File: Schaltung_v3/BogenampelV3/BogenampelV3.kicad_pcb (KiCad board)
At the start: 2 copper layers, 89 x 36 mm, 50 parts, among them IC1 TPS62742DSSR, J1 Conn_01x24_Pin, Q1 IRLML9301, Q2 IRLML6346, Q3 Si1308EDL, SW1 SW_Push, SW2 SW_Push, U1 XIAO ESP32C3

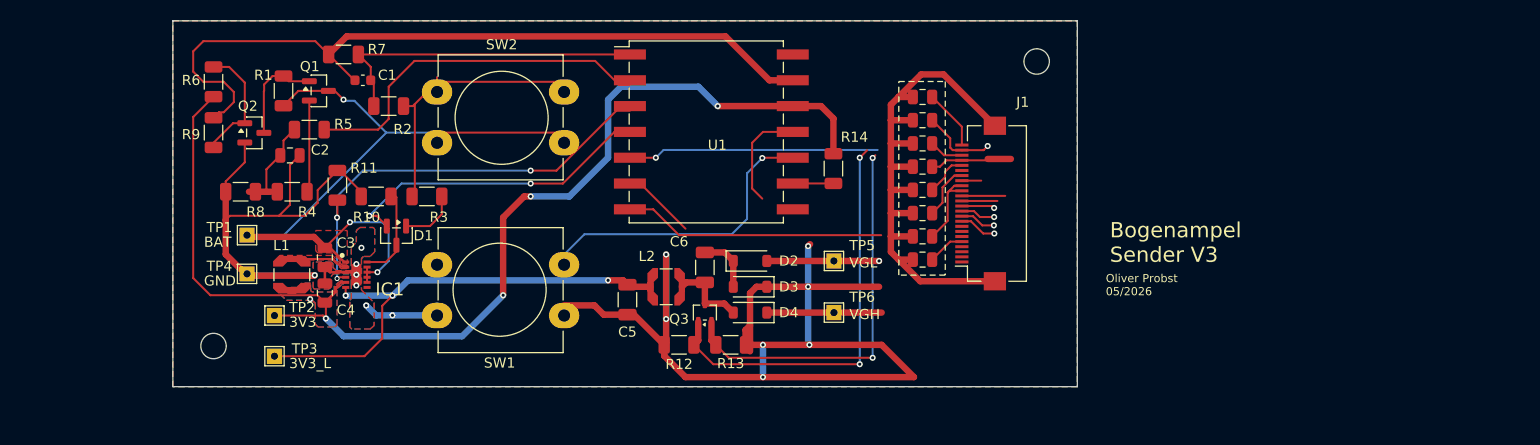
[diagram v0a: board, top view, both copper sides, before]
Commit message: Universalfernbedienung V3
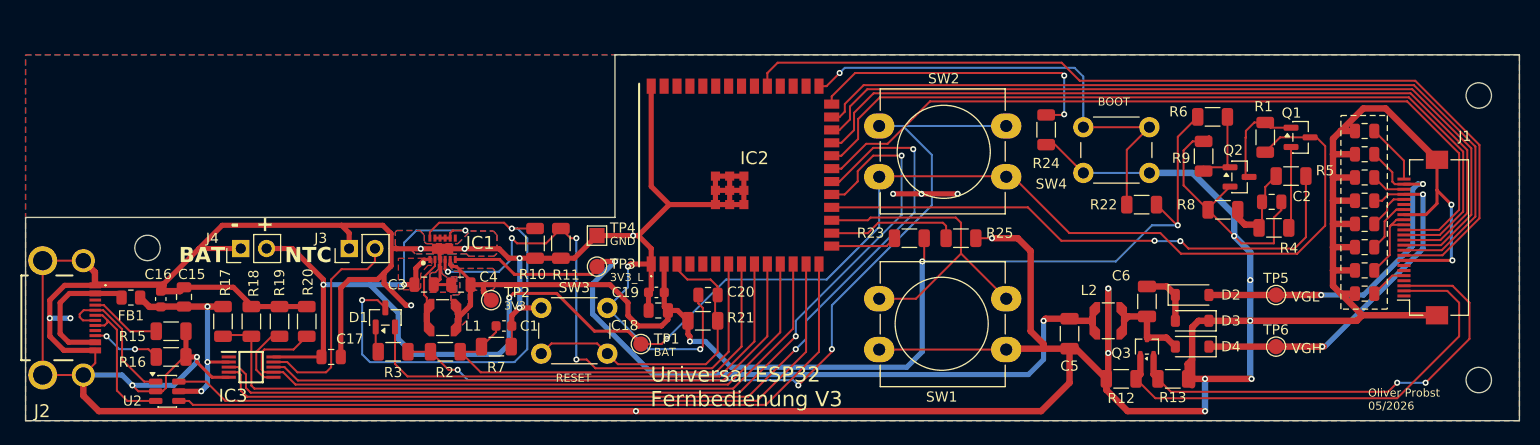
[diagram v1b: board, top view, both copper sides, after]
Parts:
- removed R14: 10k, Resistor_SMD:R_1206_3216Metric
- removed U1: XIAO ESP32C3, 0liver:xiao_esp32c3_ohneBat
- added C15: 4,7µF, Capacitor_SMD:C_0805_2012Metric, F.Cu at (81.1, 91.2)
- added C16: 100nF, Capacitor_SMD:C_0603_1608Metric, F.Cu at (78.8, 91.4)
- added C17: 4,7µF, Capacitor_SMD:C_0805_2012Metric, F.Cu at (95.6, 97.1)
- added C18: 10µF, Capacitor_SMD:C_0805_2012Metric, F.Cu at (127.8, 92.5)
- added C19: 100nF, Capacitor_SMD:C_0603_1608Metric, F.Cu at (127.6, 90.7)
- added C20: 1µF, Capacitor_SMD:C_0805_2012Metric, F.Cu at (132.7, 91.0)
- added FB1: 220, Resistor_SMD:R_0805_2012Metric, F.Cu at (75.9, 91.2)
- added IC2: ESP32-S3-WROOM-1U-N16R8, SamacSys_Parts:ESP32S3WROOM1UN16R8, F.Cu at (135.5, 79.2)
- added IC3: MCP73837T-FCI_UN, SamacSys_Parts:SOP50P490X110-10N, F.Cu at (87.7, 98.1)
- added J2: UJ20-C-H-G-MSMT-4B-P16-TR, SamacSys_Parts:UJ20CHGMSMT4BP16TR, F.Cu at (68.7, 93.2)
- added J3: NTC, Connector_PinHeader_2.54mm:PinHeader_1x02_P2.54mm_Vertical, F.Cu at (97.3, 86.4)
- added J4: BAT, Connector_PinHeader_2.54mm:PinHeader_1x02_P2.54mm_Vertical, F.Cu at (86.7, 86.4)
- added R15: 5k1, Resistor_SMD:R_1206_3216Metric, F.Cu at (79.8, 94.5)
- added R16: 5k1, Resistor_SMD:R_1206_3216Metric, F.Cu at (79.8, 97.1)
- added R17: 100k, Resistor_SMD:R_1206_3216Metric, F.Cu at (84.9, 93.6)
- added R18: 100k, Resistor_SMD:R_1206_3216Metric, F.Cu at (87.7, 93.6)
- added R19: 2k, Resistor_SMD:R_1206_3216Metric, F.Cu at (90.5, 93.6)
- added R20: 100k, Resistor_SMD:R_1206_3216Metric, F.Cu at (93.2, 93.6)
- added R21: 10k, Resistor_SMD:R_1206_3216Metric, F.Cu at (132.2, 93.5)
- added R22: 10k, Resistor_SMD:R_1206_3216Metric, F.Cu at (175.3, 82.1)
- added R23: 10k, Resistor_SMD:R_1206_3216Metric, F.Cu at (152.5, 85.4)
- added R24: 10k, Resistor_SMD:R_1206_3216Metric, F.Cu at (165.9, 74.7)
- added R25: 10k, Resistor_SMD:R_1206_3216Metric, F.Cu at (157.6, 85.4)
- added REF**: MountingHole_2.5mm, MountingHole:MountingHole_2.5mm, F.Cu at (77.5, 86.3)
- added SW3: Enable, Button_Switch_THT:SW_PUSH_6mm_H5mm, F.Cu at (116.3, 92.2)
- added SW4: Boot, Button_Switch_THT:SW_PUSH_6mm_H5mm, F.Cu at (176.1, 79.0)
- added U2: USBLC6-2SC6, Package_TO_SOT_SMD:SOT-23-6, F.Cu at (79.5, 100.5)
- TP1, TP2, TP3, TP5, TP6: footprint TestPoint:TestPoint_THTPad_1.5x1.5mm_Drill0.7mm -> TestPoint:TestPoint_Pad_D1.5mm
- TP4: footprint TestPoint:TestPoint_THTPad_1.5x1.5mm_Drill0.7mm -> TestPoint:TestPoint_Pad_1.5x1.5mm
- moved REF** 126.9 mm to (208.5, 71.3)
- moved R6 98.4 mm to (182.3, 73.5), turned to 180 degrees
- moved R9 97.5 mm to (181.4, 77.3)
- moved Q2 97.0 mm to (185.0, 79.4)
- moved R1 96.7 mm to (187.5, 75.5)
- moved C2 96.7 mm to (188.1, 81.8)
- moved Q1 96.7 mm to (191.0, 75.5)
- moved R5 96.7 mm to (190.0, 79.3)
- moved R8 96.7 mm to (183.3, 82.6)
- moved R4 96.7 mm to (188.3, 84.4)
- moved REF** 53.6 mm to (208.5, 99.3)
- moved R13 43.6 mm to (178.4, 99.2)
- moved C10 43.6 mm to (197.3, 86.3)
- moved C11 43.6 mm to (197.3, 84.0)
- moved C12 43.6 mm to (197.3, 79.4)
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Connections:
- net /GPIO_BTN1 renamed /BTN1
- net /GPIO_LOAD renamed /LOAD
- D1 pad 2: /GPIO_LATCH -> /LATCH
- J1 pad 1: /NC -> unconnected-(J1-Pin_1-Pad1)
- J1 pad 13: /SCL -> /CLK
- J1 pad 14: /SDA -> /MOSI
- J1 pad 19: /VPP -> unconnected-(J1-Pin_19-Pad19)
- J1 pad 4: /NC -> unconnected-(J1-Pin_4-Pad4)
- J1 pad 6: /TSCL -> unconnected-(J1-Pin_6-Pad6)
- J1 pad 7: /TSDA -> unconnected-(J1-Pin_7-Pad7)
- J1 pad MP: (no net) -> GND
- R5 pad 1: /ADC_BATT_SENS -> /ADC_BAT
- SW1 pad 2: /GPIO_BTN2 -> /BTN2
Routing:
- net GND: track 303.6 -> 610.6 mm, vias 14 -> 27
- net +BATT: track 73.3 -> 180.4 mm, vias 3 -> 5
- net /C_ST2: track 0.00 -> 93.6 mm, vias 0 -> 2
- net /C_ST1: track 0.00 -> 91.1 mm, vias 0 -> 2
- net /CLK: track 0.00 -> 80.6 mm
- net /BUSY: track 11.0 -> 91.3 mm, vias 1 -> 0
- net /MOSI: track 0.00 -> 78.4 mm
- net /CS_D: track 3.25 -> 81.4 mm, vias 1 -> 0
- net /USB_D+: track 0.00 -> 74.0 mm
- net /USB_D-: track 0.00 -> 73.1 mm
- net /USB_CON: track 0.00 -> 70.0 mm
- net /C_PRG: track 0.00 -> 67.3 mm
- net Net-(R2-Pad2): track 27.1 -> 89.9 mm, vias 0 -> 3
- net /C_PG: track 0.00 -> 58.1 mm
- net /ADC_BAT: track 0.00 -> 54.8 mm, vias 0 -> 2
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- removed copper zone on F.Cu, net Net-(IC1-SW)
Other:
- board size 89 x 36 mm -> 147 x 36 mm
- board text added: "+"
- board text added: "-"
- board text added: "BOOT"
- board text added: "NTC"
- board text added: "RESET"
- board text added: "Universal ESP32 Fernbedienung V3"
- board text removed: "${REFERENCE}"
- board text removed: "Bogenampel Sender V3"
